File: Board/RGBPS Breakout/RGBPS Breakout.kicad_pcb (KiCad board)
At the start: 2 copper layers, 25 x 10 mm, 11 parts, among them J1 Conn_01x04_Pin, J2 Conn_01x01_Pin

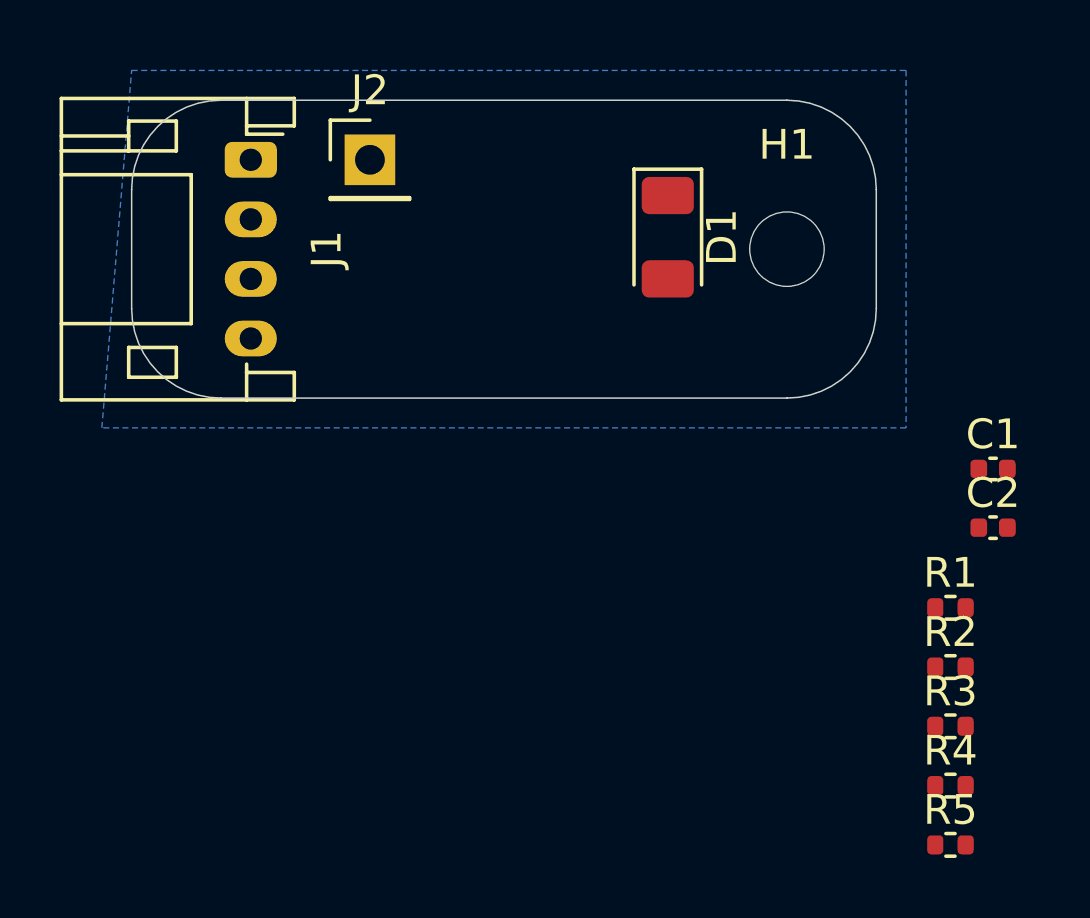
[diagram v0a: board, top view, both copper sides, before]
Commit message: routing
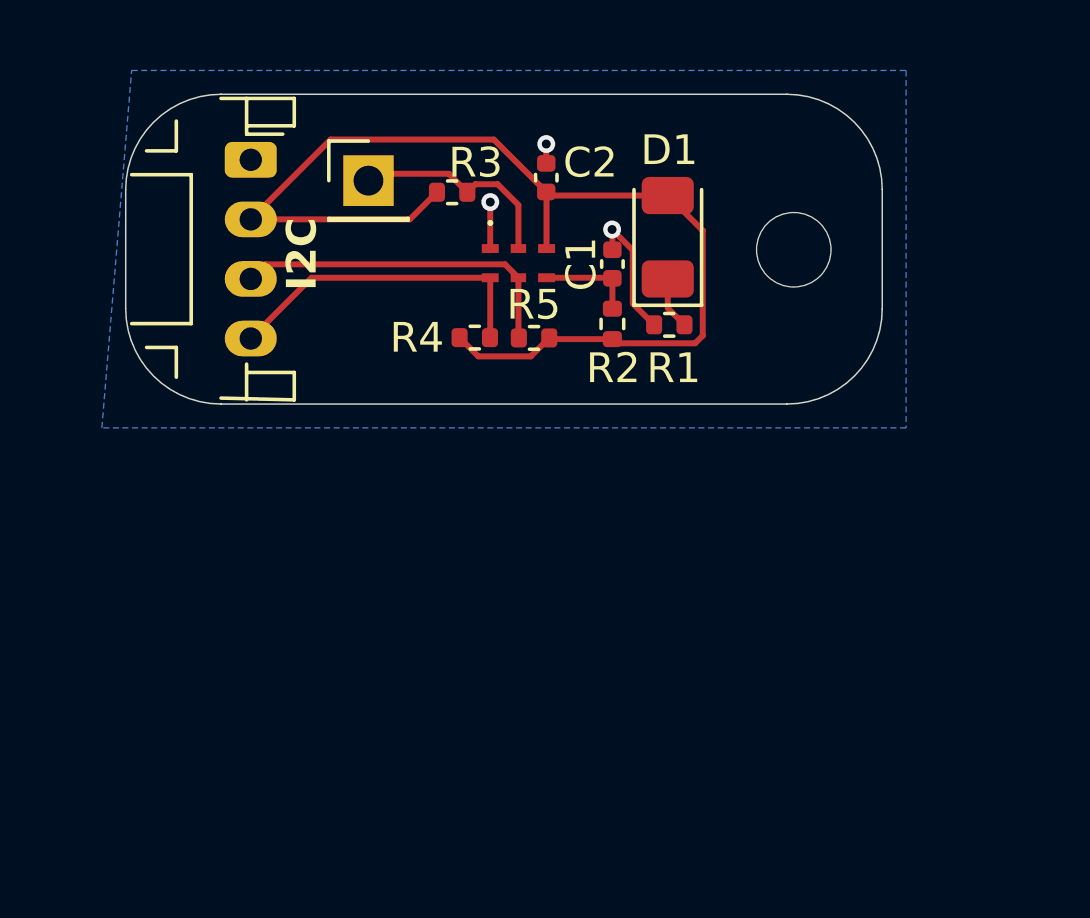
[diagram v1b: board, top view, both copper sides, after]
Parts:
- added IC1: APDS-9999, APDS-9999:APDS9999, F.Cu at (140.0, 85.5)
- D1: value 3.2V WHITE -> 2.8V WHITE
- R1: value 1.667 -> 7.7
- moved R3 24.5 mm to (137.8, 83.1), turned to 180 degrees
- moved R5 22.0 mm to (140.5, 88.0)
- moved R4 21.9 mm to (138.5, 88.0), turned to 180 degrees
- moved C2 19.1 mm to (140.9, 82.6), turned to -90 degrees
- moved R2 16.2 mm to (143.1, 87.5), turned to -90 degrees
- moved C1 14.5 mm to (143.1, 85.5), turned to 90 degrees
- moved R1 13.4 mm to (145.1, 87.5), turned to 180 degrees
- moved J2 0.70 mm to (134.9, 82.7)
- moved H1 0.23 mm to (149.2, 85.0)
- turned D1 to 90 degrees
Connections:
- D1 pad 1: +3.3V -> Net-(D1-K)
- D1 pad 2: Net-(D1-A) -> +3.3V
- R1 pad 1: Net-(D1-A) -> Net-(D1-K)
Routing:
- net +3.3V: track 0.00 -> 38.5 mm
- net SDA: track 0.00 -> 11.4 mm
- net SCL: track 0.00 -> 10.9 mm
- net INT: track 0.00 -> 7.25 mm
- net GND: track 0.00 -> 6.68 mm, vias 0 -> 3
- net Net-(IC1-VDD): track 0.00 -> 3.24 mm
- net Net-(D1-K): track 0.00 -> 1.77 mm
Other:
- board size 25 x 10 mm -> 25.4 x 10.4 mm
- board text added: "3V3"
- board text added: "GND"
- board text added: "I2C"
- board text added: "INT"
- board text added: "SCL"
- board text added: "SDA"
